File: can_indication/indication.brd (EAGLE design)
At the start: 98.7 x 50.8 mm, 33 parts, among them CON1 SM04B-GHS-TB, CON2 SM04B-GHS-TB, IC1 TPS92630QPWPRQ1, IC2 TPS92630QPWPRQ1, U1 STM32F103CB

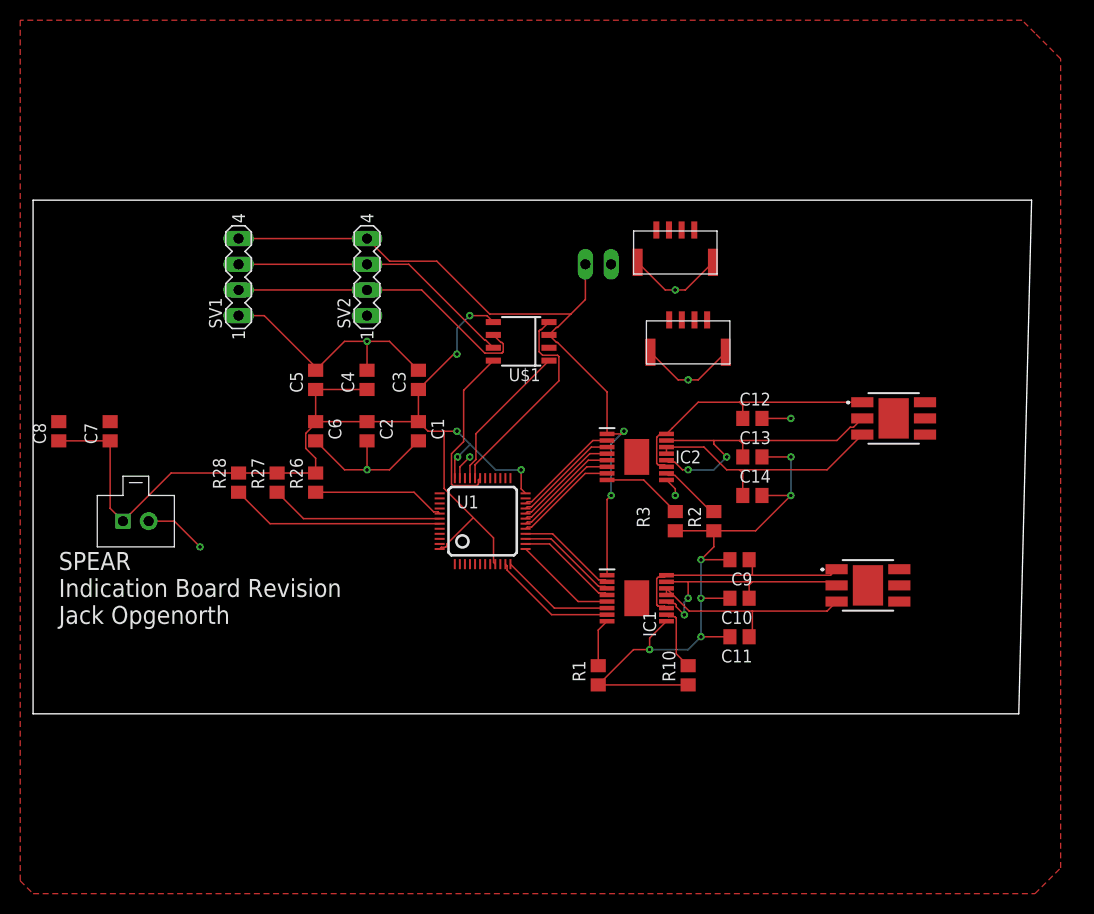
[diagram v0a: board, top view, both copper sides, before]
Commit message: Fixed everything that needed to be fixed (hopefully)
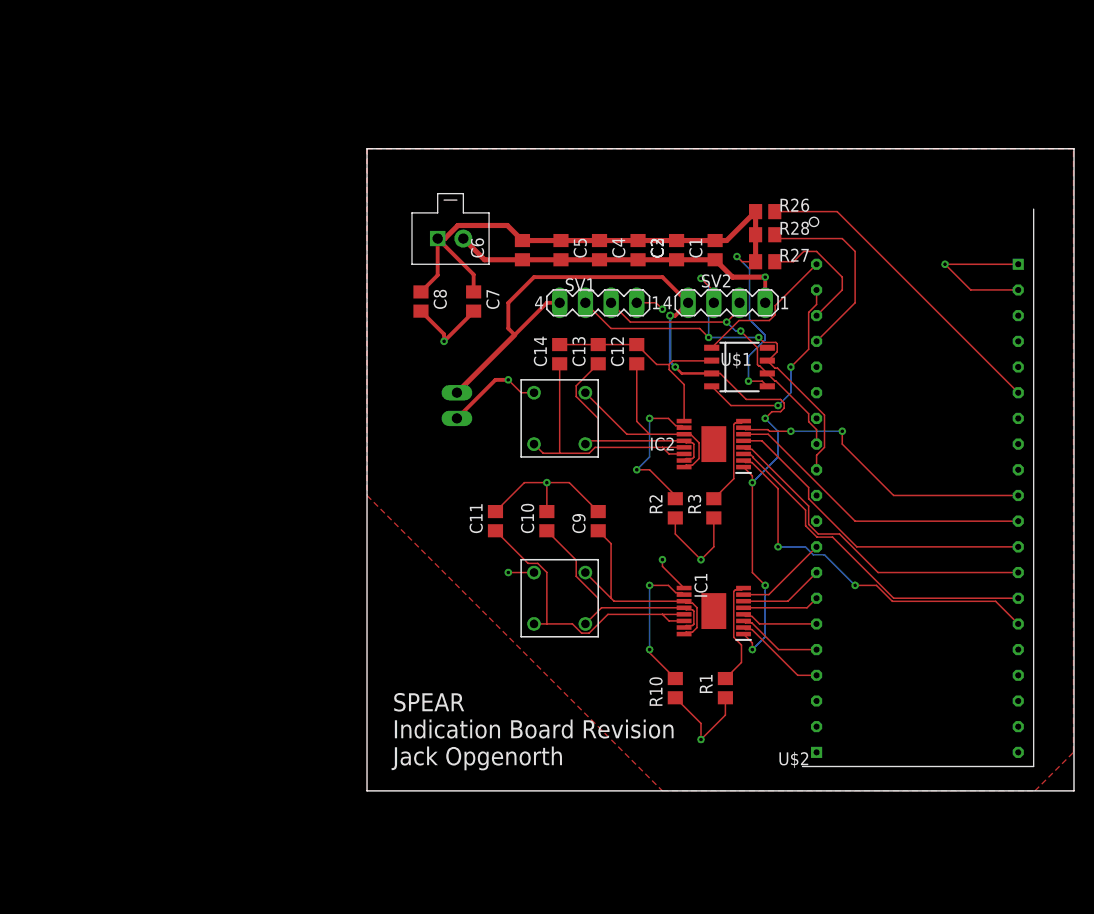
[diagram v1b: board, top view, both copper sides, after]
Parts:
- removed CON1, CON2: SM04B-GHS-TB, ARVP:SM04B-GHS-TB
- removed LED1, LED2: AAAF5051-05, AAAF5051-05:AAAF505105
- removed U1: STM32F103CB, SPEAR:LQFP48
- added U$2: STM-DEV-BOARD, SPEAR:STM-DEV-BOARD
- added U$3, U$5: R50RGB-4-0045, SPEAR-indication:R50RGB-4-0045
- C10, C11, C12, C13, C14, C9: value (none) -> 100n
- moved R28 57.6 mm to (72.4, 62.6), turned to 180 degrees
- moved R27 53.0 mm to (72.4, 59.9), turned to 180 degrees
- moved R26 51.9 mm to (72.4, 64.9), turned to 180 degrees
- moved U$4 41.8 mm to (41.3, 62.2)
- moved C7 38.2 mm to (43.6, 56.0), turned to 270 degrees
- moved C8 38.0 mm to (38.4, 56.0), turned to 270 degrees
- moved SV1 35.7 mm to (55.9, 55.9), turned to 180 degrees
- moved SV2 35.7 mm to (68.6, 55.9), turned to 180 degrees
- moved C2 35.5 mm to (63.6, 61.1)
- moved C1 34.4 mm to (67.4, 61.1)
- moved C5 27.4 mm to (52.2, 61.1), turned to 270 degrees
- moved C6 27.2 mm to (48.4, 61.1)
- moved C11 26.7 mm to (45.7, 34.3), turned to 90 degrees
- moved C4 26.3 mm to (56.0, 61.1), turned to 270 degrees
- moved C3 25.2 mm to (59.8, 61.1), turned to 270 degrees
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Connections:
- removed net BOOT0: U1.44
- removed net N$14: U1.46
- removed net NRST: U1.7
- removed net PA7: IC2.7, U1.17
- removed net PB0: IC2.6, U1.18
- removed net PB1: IC2.5, U1.19
- removed net PB10: IC2.3, U1.21
- removed net PB11: IC2.2, U1.22
- removed net PB2: IC2.4, U1.20
- removed net SWCLK: U1.37
- removed net SWDIO: U1.34
- new net PB4: IC1.7, U$2.PB4
- new net PB5: IC1.6, U$2.PB5
- new net PB6: IC1.5, U$2.PB6
- new net PB7: IC1.4, U$2.PB7
- new net PB9: IC1.2, U$2.PB9
- net +3V3: no longer U1.24, U1.36, U1.48, U1.9
- net CANH: now also U$2.CANH
- net CANL: now also U$2.CANL
- net CAN_STBY: no longer U1.31
- net GND: now also U$2.GND@2, U$2.GND@3, U$3.P$2, U$5.P$2; no longer CON1.P$5, CON1.P$6, CON2.P$5, CON2.P$6, U1.23, U1.35, U1.47, U1.8
- net I2C_SCL: now also U$2.PB14; no longer U1.42
- net I2C_SDA: now also U$2.PB15; no longer U1.43
- net L1OUT1: now also U$3.P$3; no longer LED1.1
- net L1OUT2: now also U$3.P$4; no longer LED1.2
- net L1OUT3: now also U$3.P$1; no longer LED1.3
- net L2OUT1: now also U$5.P$3; no longer LED2.1
- net L2OUT2: now also U$5.P$4; no longer LED2.2
- net L2OUT3: now also U$5.P$1; no longer LED2.3
- net LED_!OE: now also U$2.PB10; no longer U1.41
- net PA1: now also IC2.2, U$2.PA1; no longer IC1.7, U1.11
- net PA2: now also IC2.3, U$2.PA2; no longer IC1.6, U1.12
- net PA3: now also IC2.4, U$2.PA3; no longer IC1.5, U1.13
- net PA4: now also IC2.5, U$2.PA4; no longer IC1.4, U1.14
- net PA5: now also IC2.6, U$2.PA5; no longer IC1.3, U1.15
- net PA6: now also IC2.7, U$2.PA6; no longer IC1.2, U1.16
- net PB8: now also IC1.3, U$2.PB8; no longer U1.45
- net STM_CANRX: now also U$2.PB13; no longer U1.32
- net STM_CANTX: now also U$2.PB12; no longer U1.33
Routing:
- net +3V3: track 112.8 -> 69.7 mm, vias 5 -> 2
- net PA1: track 12.4 -> 37.2 mm, vias 0 -> 2
- net PA3: track 10.2 -> 33.4 mm
- net PA2: track 11.4 -> 34.0 mm
- net PA4: track 10.1 -> 32.2 mm
- net PA6: track 10.0 -> 30.7 mm, vias 0 -> 2
- net PA5: track 10.1 -> 30.7 mm
- net LED_!OE: track 13.1 -> 31.5 mm
- net CAN_STBY: track 17.4 -> 0.00 mm
- net CANH: track 28.6 -> 45.6 mm, vias 0 -> 3
- net +5V: track 73.4 -> 89.1 mm, vias 2 -> 6
- net PB11: track 10.6 -> 0.00 mm
- net PB10: track 10.6 -> 0.00 mm
- net PB2: track 10.5 -> 0.00 mm
- net PB1: track 10.4 -> 0.00 mm
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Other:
- board size 98.7 x 50.8 mm -> 69.9 x 63.5 mm
